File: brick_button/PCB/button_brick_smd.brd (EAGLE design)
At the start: 23.2 x 29.5 mm, 3 parts

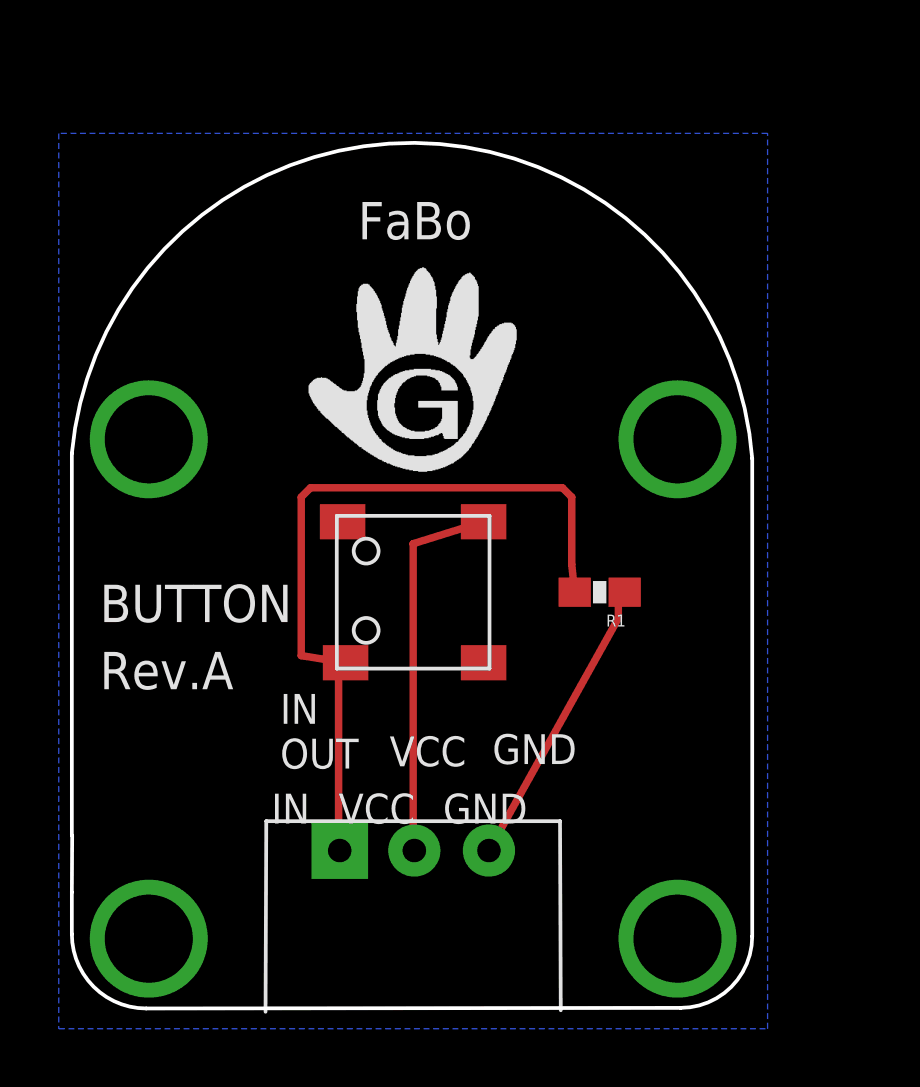
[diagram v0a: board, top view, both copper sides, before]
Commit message: refine PCB board fix library
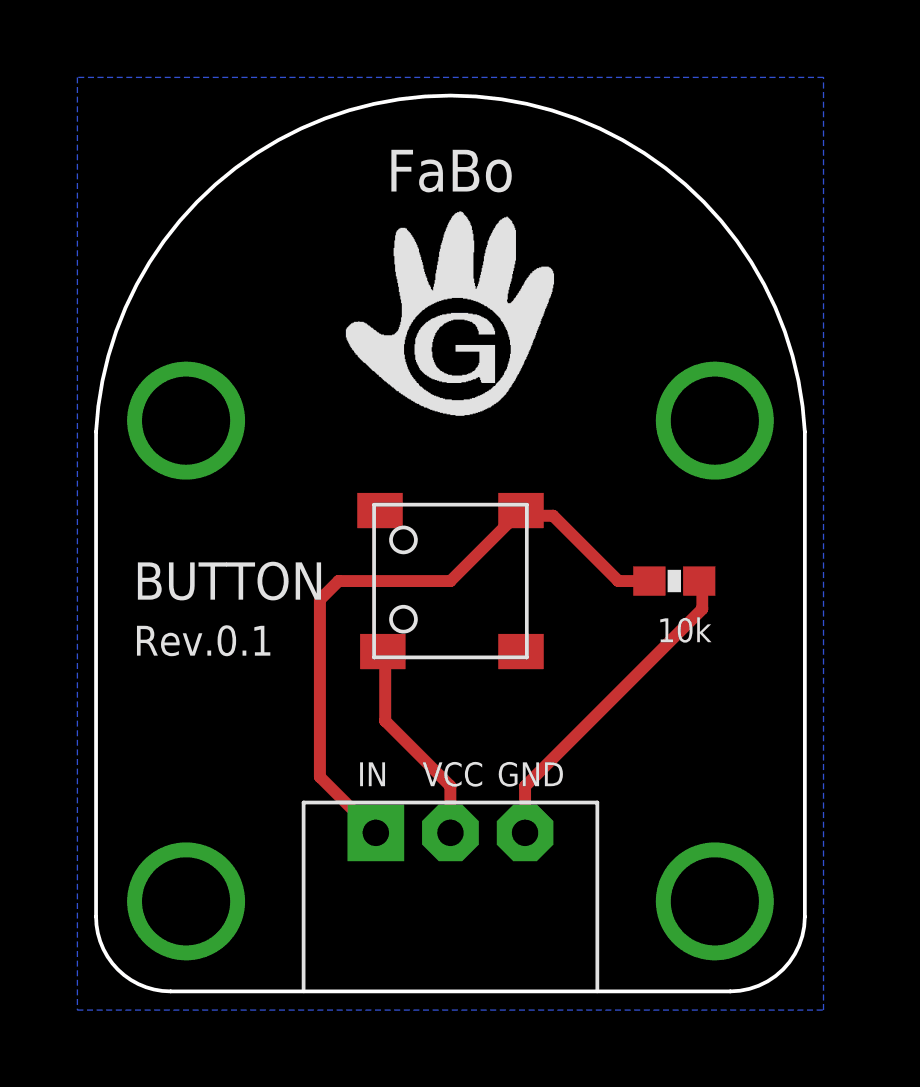
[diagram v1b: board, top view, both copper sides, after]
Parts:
- removed U$1: BRICK-3PIN, gclue:BRICK_3PIN
- removed U$2: SWITCH-LS6J2M-T, gclue:SWICTH-LS6J2M-T
- added J1: BRICK_3PIN, gclue:BRICK_3PIN
- added S1: SWITCH-LS6J2M-T, gclue:SWITCH-LS6J2M-T
- R1: value (none) -> 10k; device SparkFun:0603-RES -> SparkFun-Resistors:0603-RES
- moved R1 2.57 mm to (20.3, 14.6)
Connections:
- removed net N$2: R1.2, U$1.IN/OUT, U$2.2
- new net N$1: J1.VCC, S1.2
- net GND: now also J1.GND; no longer U$1.GND
- net N$3: now also J1.IN/OUT, R1.2, S1.3; no longer U$1.VCC, U$2.3
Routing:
- net N$2: track 26.3 -> 0.00 mm
- net N$3: track 13.0 -> 22.2 mm
- net N$1: track 0.00 -> 7.13 mm
- net GND: track 10.2 -> 11.1 mm
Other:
- board size 23.2 x 29.5 mm -> 24.1 x 30.5 mm
- board text added: "Rev.0.1"
- board text removed: "Rev.A"
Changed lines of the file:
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@@
 <layer number="56" name="wert" color="7" fill="1" visible="no" active="no"/>
 <layer number="57" name="tCAD" color="7" fill="1" visible="no" active="no"/>
+<layer number="90" name="Modules" color="5" fill="1" visible="no" active="no"/>
 <layer number="91" name="Nets" color="2" fill="1" visible="no" active="no"/>
 <layer number="92" name="Busses" color="1" fill="1" visible="no" active="no"/>
@@
 <layer number="97" name="Info" color="7" fill="1" visible="no" active="no"/>
 <layer number="98" name="Guide" color="6" fill="1" visible="no" active="no"/>
+<layer number="99" name="SpiceOrder" color="7" fill="1" visible="no" active="no"/>
 <layer number="100" name="Muster" color="7" fill="1" visible="no" active="no"/>
 <layer number="101" name="Patch_Top" color="12" fill="4" visible="no" active="yes"/>
@@
 <layer number="111" name="LPC17xx" color="7" fill="1" visible="yes" active="yes"/>
 <layer number="112" name="tSilk" color="7" fill="1" visible="yes" active="yes"/>
+<layer number="113" name="IDFDebug" color="4" fill="1" visible="yes" active="yes"/>
 <layer number="116" name="Patch_BOT" color="9" fill="4" visible="no" active="yes"/>
 <layer number="121" name="_tsilk" color="7" fill="1" visible="no" active="yes"/>
@@
 <board>
 <plain>
-<text x="8.89" y="6.35" size="1.016" layer="21">VCC</text>
-<text x="12.446" y="6.35" size="1.016" layer="21">GND</text>
-<text x="6.604" y="6.35" size="1.016" layer="21">IN</text>
-<text x="0.762" y="13.208" size="1.27" layer="21">BUTTON</text>
-<text x="0.762" y="10.922" size="1.27" layer="21">Rev.A</text>
+<text x="11.7475" y="7.62" size="0.8128" layer="21" font="vector">VCC</text>
+<text x="14.2875" y="7.62" size="0.8128" layer="21" font="vector">GND</text>
+<text x="9.525" y="7.62" size="0.8128" layer="21" font="vector">IN</text>
+<text x="1.905" y="13.97" size="1.27" layer="21" font="vector">BUTTON</text>
+<text x="1.905" y="12.065" size="1.016" layer="21" font="vector">Rev.0.1</text>
 </plain>
 <attributes>
@@
 </autorouter>
 <elements>
-<element name="R1" library="SparkFun" package="0603-RES" value="" x="17.78" y="14.224" smashed="yes" rot="R180">
-<attribute name="NAME" x="18.669" y="13.462" size="0.4064" layer="25" font="vector" rot="R180"/>
-<attribute name="VALUE" x="18.796" y="15.367" size="0.4064" layer="27" font="vector" rot="R180"/>
+<element name="S1" library="gclue" package="SWITCH-LS6J2M-T" value="SWITCH-LS6J2M-T" x="12.7" y="14.605" smashed="yes"/>
+<element name="R1" library="SparkFun-Resistors" package="0603-RES" value="10k" x="20.32" y="14.605" smashed="yes" rot="R180">
+<attribute name="VALUE" x="21.59" y="13.335" size="0.8128" layer="21" font="vector" rot="R180"/>
 </element>
-<element name="U$1" library="gclue" package="BRICK_3PIN" value="BRICK-3PIN" x="11.43" y="11.43"/>
-<element name="U$2" library="gclue" package="SWICTH-LS6J2M-T" value="SWITCH-LS6J2M-T" x="11.43" y="14.224"/>
+<element name="J1" library="gclue" package="BRICK_3PIN" value="BRICK_3PIN" x="12.7" y="14.605"/>
 </elements>
 <signals>
 <signal name="GND">
-<contactref element="U$1" pad="GND"/>
+<contactref element="J1" pad="GND"/>
 <contactref element="R1" pad="1"/>
-<wire x1="18.63" y1="14.224" x2="18.415" y2="14.224" width="0.254" layer="1"/>
-<wire x1="18.415" y1="14.224" x2="18.415" y2="13.335" width="0.254" layer="1"/>
-<wire x1="18.415" y1="13.335" x2="14.01" y2="5.43" width="0.254" layer="1"/>
+<wire x1="15.24" y1="6.0325" x2="15.24" y2="7.62" width="0.4064" layer="1"/>
+<wire x1="15.24" y1="7.62" x2="21.2725" y2="13.6525" width="0.4064" layer="1"/>
+<wire x1="21.2725" y1="13.6525" x2="21.2725" y2="14.5025" width="0.4064" layer="1"/>
+<wire x1="21.2725" y1="14.5025" x2="21.17" y2="14.605" width="0.4064" layer="1"/>
 <polygon width="0.254" layer="16">
-<vertex x="-0.635" y="-0.635"/>
-<vertex x="23.495" y="-0.635"/>
-<vertex x="23.495" y="29.845"/>
-<vertex x="-0.635" y="29.845"/>
+<vertex x="0" y="0"/>
+<vertex x="25.4" y="0"/>
+<vertex x="25.4" y="31.75"/>
+<vertex x="0" y="31.75"/>
 </polygon>
 </signal>
-<signal name="N$2">
-<contactref element="R1" pad="2"/>
-<contactref element="U$2" pad="2"/>
-<contactref element="U$1" pad="IN/OUT"/>
-<wire x1="8.93" y1="5.43" x2="8.89" y2="5.43" width="0.254" layer="1"/>
-<wire x1="8.89" y1="5.43" x2="8.89" y2="5.715" width="0.254" layer="1"/>
-<wire x1="8.89" y1="5.715" x2="8.89" y2="11.43" width="0.254" layer="1"/>
-<wire x1="8.89" y1="11.43" x2="8.89" y2="11.824" width="0.254" layer="1"/>
-<wire x1="8.89" y1="11.824" x2="9.13" y2="11.824" width="0.254" layer="1"/>
-<wire x1="9.13" y1="11.824" x2="7.62" y2="12.065" width="0.254" layer="1"/>
-<wire x1="7.62" y1="12.065" x2="7.62" y2="17.4625" width="0.254" layer="1"/>
-<wire x1="7.62" y1="17.4625" x2="7.9375" y2="17.78" width="0.254" layer="1"/>
-<wire x1="7.9375" y1="17.78" x2="16.51" y2="17.78" width="0.254" layer="1"/>
-<wire x1="16.51" y1="17.78" x2="16.8275" y2="17.4625" width="0.254" layer="1"/>
-<wire x1="16.8275" y1="17.4625" x2="16.8275" y2="15.1765" width="0.254" layer="1"/>
-<wire x1="16.8275" y1="15.1765" x2="16.93" y2="14.224" width="0.254" layer="1"/>
+<signal name="N$1">
+<contactref element="J1" pad="VCC"/>
+<contactref element="S1" pad="2"/>
+<wire x1="12.7" y1="6.0325" x2="12.7" y2="7.62" width="0.4064" layer="1"/>
+<wire x1="12.7" y1="7.62" x2="10.4775" y2="9.8425" width="0.4064" layer="1"/>
+<wire x1="10.4775" y1="9.8425" x2="10.4775" y2="12.1275" width="0.4064" layer="1"/>
+<wire x1="10.4775" y1="12.1275" x2="10.4" y2="12.205" width="0.4064" layer="1"/>
 </signal>
 <signal name="N$3">
-<contactref element="U$1" pad="VCC"/>
-<contactref element="U$2" pad="3"/>
-<wire x1="13.83" y1="16.624" x2="11.43" y2="15.875" width="0.254" layer="1"/>
-<wire x1="11.43" y1="15.875" x2="11.43" y2="5.715" width="0.254" layer="1"/>
-<wire x1="11.43" y1="5.715" x2="11.43" y2="5.43" width="0.254" layer="1"/>
-<wire x1="11.43" y1="5.43" x2="11.47" y2="5.43" width="0.254" layer="1"/>
+<contactref element="R1" pad="2"/>
+<contactref element="S1" pad="3"/>
+<contactref element="J1" pad="IN/OUT"/>
+<wire x1="19.47" y1="14.605" x2="18.415" y2="14.605" width="0.4064" layer="1"/>
+<wire x1="18.415" y1="14.605" x2="16.1925" y2="16.8275" width="0.4064" layer="1"/>
+<wire x1="16.1925" y1="16.8275" x2="15.2775" y2="16.8275" width="0.4064" layer="1"/>
+<wire x1="15.2775" y1="16.8275" x2="15.1" y2="17.005" width="0.4064" layer="1"/>
+<wire x1="15.1" y1="17.005" x2="12.7" y2="14.605" width="0.4064" layer="1"/>
+<wire x1="12.7" y1="14.605" x2="8.89" y2="14.605" width="0.4064" layer="1"/>
+<wire x1="8.89" y1="14.605" x2="8.255" y2="13.97" width="0.4064" layer="1"/>
+<wire x1="8.255" y1="13.97" x2="8.255" y2="7.9375" width="0.4064" layer="1"/>
+<wire x1="8.255" y1="7.9375" x2="10.16" y2="6.0325" width="0.4064" layer="1"/>
 </signal>
 </signals>
 </board>
 </drawing>
-<compatibility>
-<note version="6.3" minversion="6.2.2" severity="warning">
-Since Version 6.2.2 text objects can contain more than one line,
-which will not be processed correctly with this version.
-</note>
-</compatibility>
 </eagle>

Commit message: Refine boards
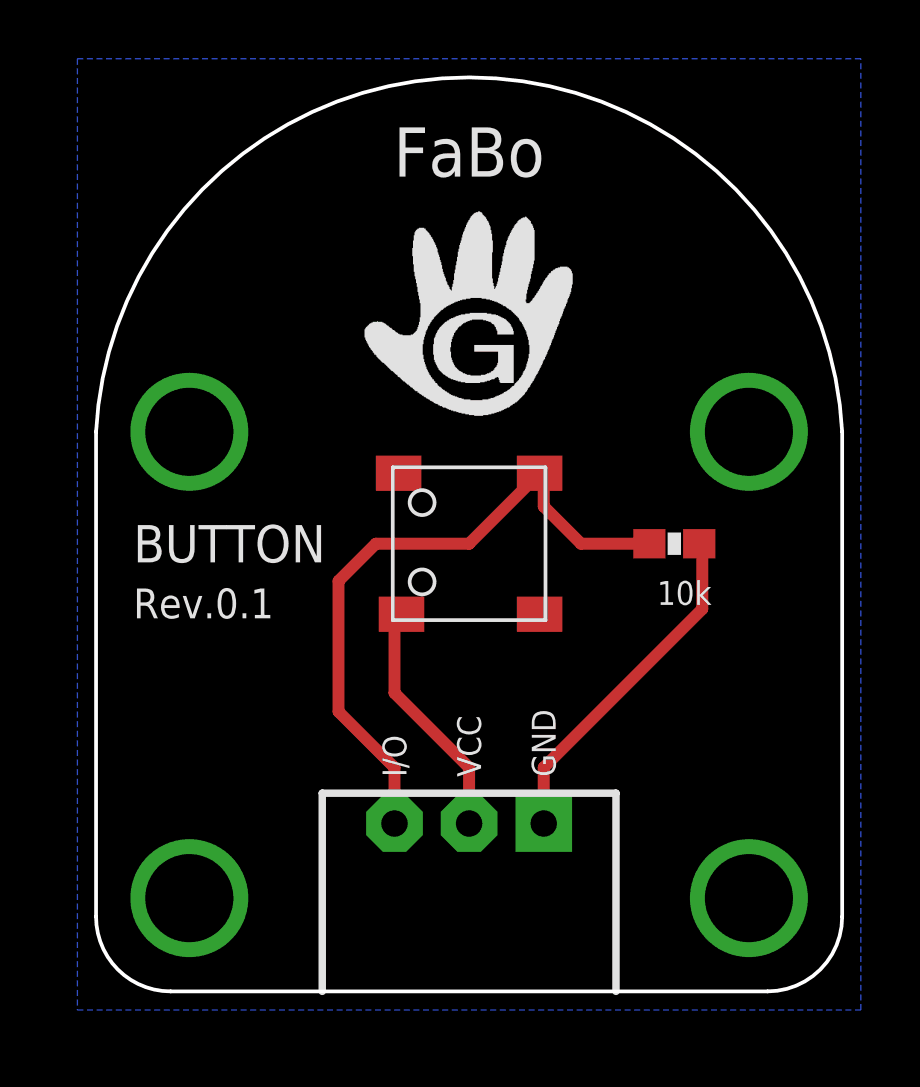
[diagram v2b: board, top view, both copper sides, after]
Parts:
- moved J1 1.42 mm to (13.3, 15.9)
- moved S1 1.42 mm to (13.3, 15.9)
- moved R1 1.27 mm to (20.3, 15.9)
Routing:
- net N$1: track 7.13 -> 8.31 mm
- net GND: track 11.1 -> 11.8 mm
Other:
- board size 24.1 x 30.5 mm -> 25.4 x 31.1 mm
- board text removed: "GND"
- board text removed: "IN"
- board text removed: "VCC"
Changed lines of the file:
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@@
 <board>
 <plain>
-<text x="11.7475" y="7.62" size="0.8128" layer="21" font="vector">VCC</text>
-<text x="14.2875" y="7.62" size="0.8128" layer="21" font="vector">GND</text>
-<text x="9.525" y="7.62" size="0.8128" layer="21" font="vector">IN</text>
-<text x="1.905" y="13.97" size="1.27" layer="21" font="vector">BUTTON</text>
-<text x="1.905" y="12.065" size="1.016" layer="21" font="vector">Rev.0.1</text>
+<text x="1.905" y="15.24" size="1.27" layer="21" font="vector">BUTTON</text>
+<text x="1.905" y="13.335" size="1.016" layer="21" font="vector">Rev.0.1</text>
 </plain>
 <attributes>
@@
 </autorouter>
 <elements>
-<element name="S1" library="gclue" package="SWITCH-LS6J2M-T" value="SWITCH-LS6J2M-T" x="12.7" y="14.605" smashed="yes"/>
-<element name="R1" library="SparkFun-Resistors" package="0603-RES" value="10k" x="20.32" y="14.605" smashed="yes" rot="R180">
-<attribute name="VALUE" x="21.59" y="13.335" size="0.8128" layer="21" font="vector" rot="R180"/>
+<element name="S1" library="gclue" package="SWITCH-LS6J2M-T" value="SWITCH-LS6J2M-T" x="13.335" y="15.875" smashed="yes"/>
+<element name="R1" library="SparkFun-Resistors" package="0603-RES" value="10k" x="20.32" y="15.875" smashed="yes" rot="R180">
+<attribute name="VALUE" x="21.59" y="14.605" size="0.8128" layer="21" font="vector" rot="R180"/>
 </element>
-<element name="J1" library="gclue" package="BRICK_3PIN" value="BRICK_3PIN" x="12.7" y="14.605"/>
+<element name="J1" library="gclue" package="BRICK_3PIN" value="BRICK_3PIN" x="13.335" y="15.875"/>
 </elements>
 <signals>
@@
 <contactref element="J1" pad="GND"/>
 <contactref element="R1" pad="1"/>
-<wire x1="15.24" y1="6.0325" x2="15.24" y2="7.62" width="0.4064" layer="1"/>
-<wire x1="15.24" y1="7.62" x2="21.2725" y2="13.6525" width="0.4064" layer="1"/>
-<wire x1="21.2725" y1="13.6525" x2="21.2725" y2="14.5025" width="0.4064" layer="1"/>
-<wire x1="21.2725" y1="14.5025" x2="21.17" y2="14.605" width="0.4064" layer="1"/>
-<polygon width="0.254" layer="16">
+<wire x1="15.875" y1="6.35" x2="15.875" y2="8.255" width="0.4064" layer="1"/>
+<wire x1="15.875" y1="8.255" x2="21.2725" y2="13.6525" width="0.4064" layer="1"/>
+<wire x1="21.2725" y1="13.6525" x2="21.2725" y2="15.7725" width="0.4064" layer="1"/>
+<wire x1="21.2725" y1="15.7725" x2="21.17" y2="15.875" width="0.4064" layer="1"/>
+<polygon width="0.254" layer="16" spacing="1.016">
 <vertex x="0" y="0"/>
-<vertex x="25.4" y="0"/>
-<vertex x="25.4" y="31.75"/>
-<vertex x="0" y="31.75"/>
+<vertex x="26.67" y="0"/>
+<vertex x="26.67" y="32.385"/>
+<vertex x="0" y="32.385"/>
 </polygon>
 </signal>
@@
 <contactref element="J1" pad="VCC"/>
 <contactref element="S1" pad="2"/>
-<wire x1="12.7" y1="6.0325" x2="12.7" y2="7.62" width="0.4064" layer="1"/>
-<wire x1="12.7" y1="7.62" x2="10.4775" y2="9.8425" width="0.4064" layer="1"/>
-<wire x1="10.4775" y1="9.8425" x2="10.4775" y2="12.1275" width="0.4064" layer="1"/>
-<wire x1="10.4775" y1="12.1275" x2="10.4" y2="12.205" width="0.4064" layer="1"/>
+<wire x1="13.335" y1="6.35" x2="13.335" y2="8.255" width="0.4064" layer="1"/>
+<wire x1="13.335" y1="8.255" x2="10.795" y2="10.795" width="0.4064" layer="1"/>
+<wire x1="10.795" y1="10.795" x2="10.795" y2="13.335" width="0.4064" layer="1"/>
+<wire x1="10.795" y1="13.335" x2="11.035" y2="13.475" width="0.4064" layer="1"/>
 </signal>
 <signal name="N$3">
@@
 <contactref element="S1" pad="3"/>
 <contactref element="J1" pad="IN/OUT"/>
-<wire x1="19.47" y1="14.605" x2="18.415" y2="14.605" width="0.4064" layer="1"/>
-<wire x1="18.415" y1="14.605" x2="16.1925" y2="16.8275" width="0.4064" layer="1"/>
-<wire x1="16.1925" y1="16.8275" x2="15.2775" y2="16.8275" width="0.4064" layer="1"/>
-<wire x1="15.2775" y1="16.8275" x2="15.1" y2="17.005" width="0.4064" layer="1"/>
-<wire x1="15.1" y1="17.005" x2="12.7" y2="14.605" width="0.4064" layer="1"/>
-<wire x1="12.7" y1="14.605" x2="8.89" y2="14.605" width="0.4064" layer="1"/>
-<wire x1="8.89" y1="14.605" x2="8.255" y2="13.97" width="0.4064" layer="1"/>
-<wire x1="8.255" y1="13.97" x2="8.255" y2="7.9375" width="0.4064" layer="1"/>
-<wire x1="8.255" y1="7.9375" x2="10.16" y2="6.0325" width="0.4064" layer="1"/>
+<wire x1="19.47" y1="15.875" x2="17.145" y2="15.875" width="0.4064" layer="1"/>
+<wire x1="17.145" y1="15.875" x2="15.875" y2="17.145" width="0.4064" layer="1"/>
+<wire x1="15.875" y1="17.145" x2="15.875" y2="17.78" width="0.4064" layer="1"/>
+<wire x1="15.875" y1="17.78" x2="15.735" y2="18.275" width="0.4064" layer="1"/>
+<wire x1="15.735" y1="18.275" x2="13.335" y2="15.875" width="0.4064" layer="1"/>
+<wire x1="13.335" y1="15.875" x2="10.16" y2="15.875" width="0.4064" layer="1"/>
+<wire x1="10.16" y1="15.875" x2="8.89" y2="14.605" width="0.4064" layer="1"/>
+<wire x1="8.89" y1="14.605" x2="8.89" y2="10.16" width="0.4064" layer="1"/>
+<wire x1="8.89" y1="10.16" x2="10.795" y2="8.255" width="0.4064" layer="1"/>
+<wire x1="10.795" y1="8.255" x2="10.795" y2="6.35" width="0.4064" layer="1"/>
 </signal>
 </signals>
